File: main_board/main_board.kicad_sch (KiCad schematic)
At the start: 68 parts, among them J1 3.5mm Jack, J18 Conn_01x15_Female, J19 Conn_01x15_Female, J2 3.5mm Jack, J3 3.5mm Jack, J4 3.5mm Jack, J5 Display Header, J6 EU Power, J7 Expansion Header, SW1 Push Button, SW10 Push Button, SW11 Push Button, SW12 Push Button, SW13 Push Button, SW14 Push Button, SW15 Push Button, SW16 Push Button, SW17 Push Button, SW2 Push Button, SW3 Push Button, SW4 Push Button, SW5 Adj, SW6 Push Button, SW7 Push Button, SW8 Push Button, SW9 Push Button, U14 MCP23008-xSO, U3 CD4013BPWR, U4 CD4013BPWR

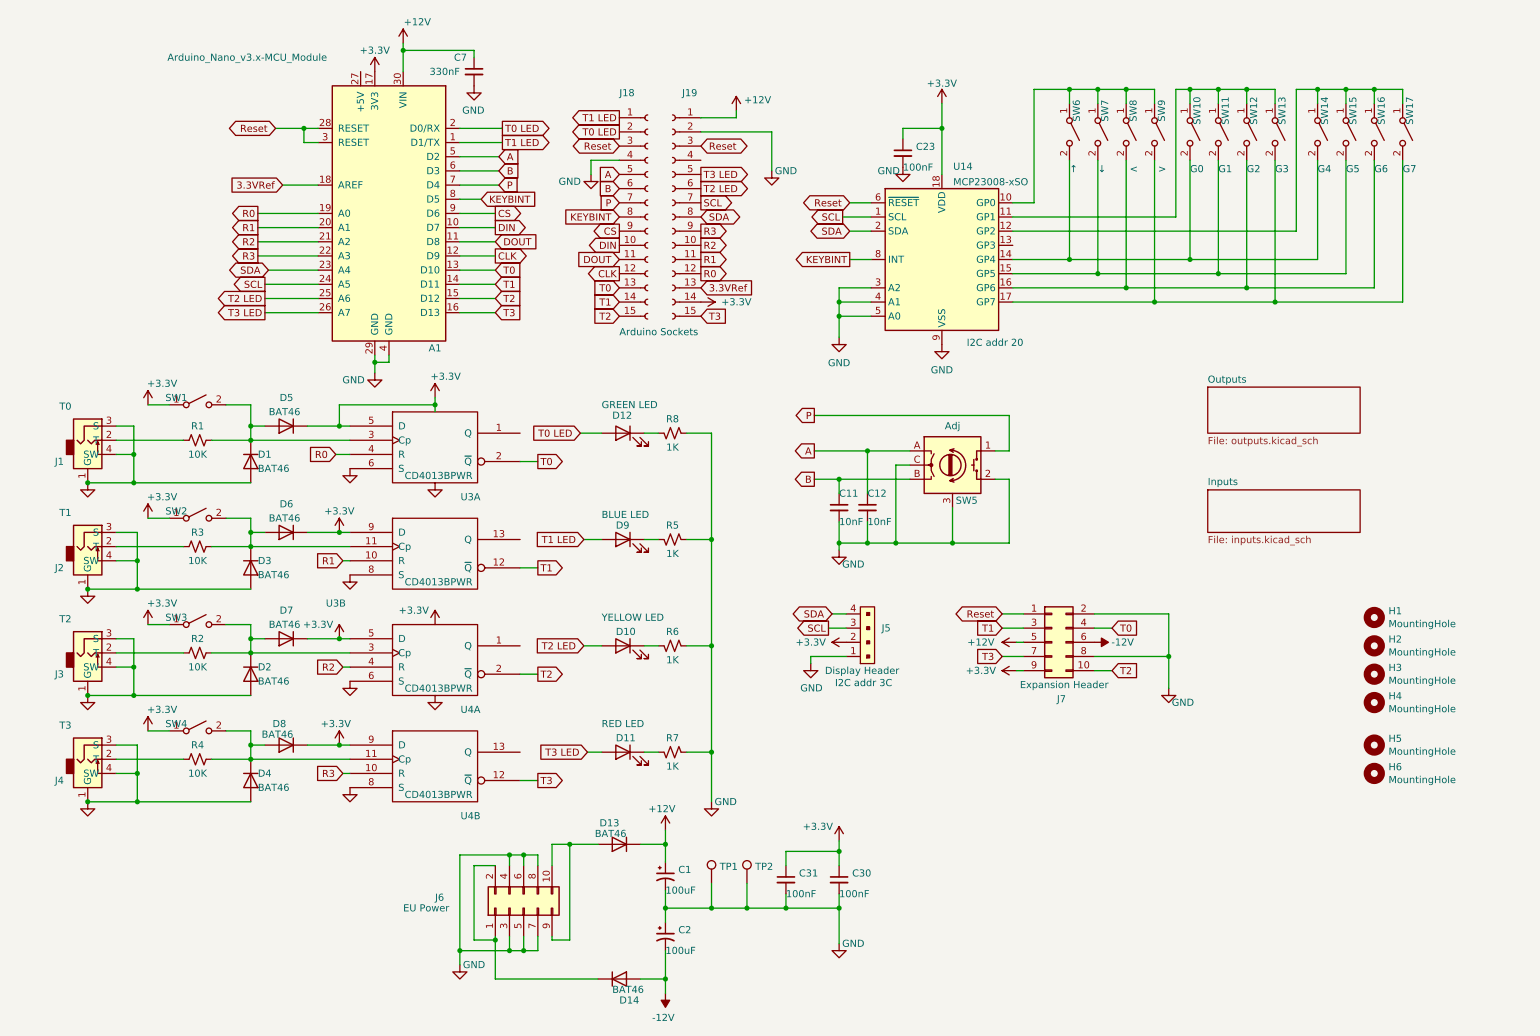
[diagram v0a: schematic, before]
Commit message: Ver 2.0 of board.
Also major advances in code.
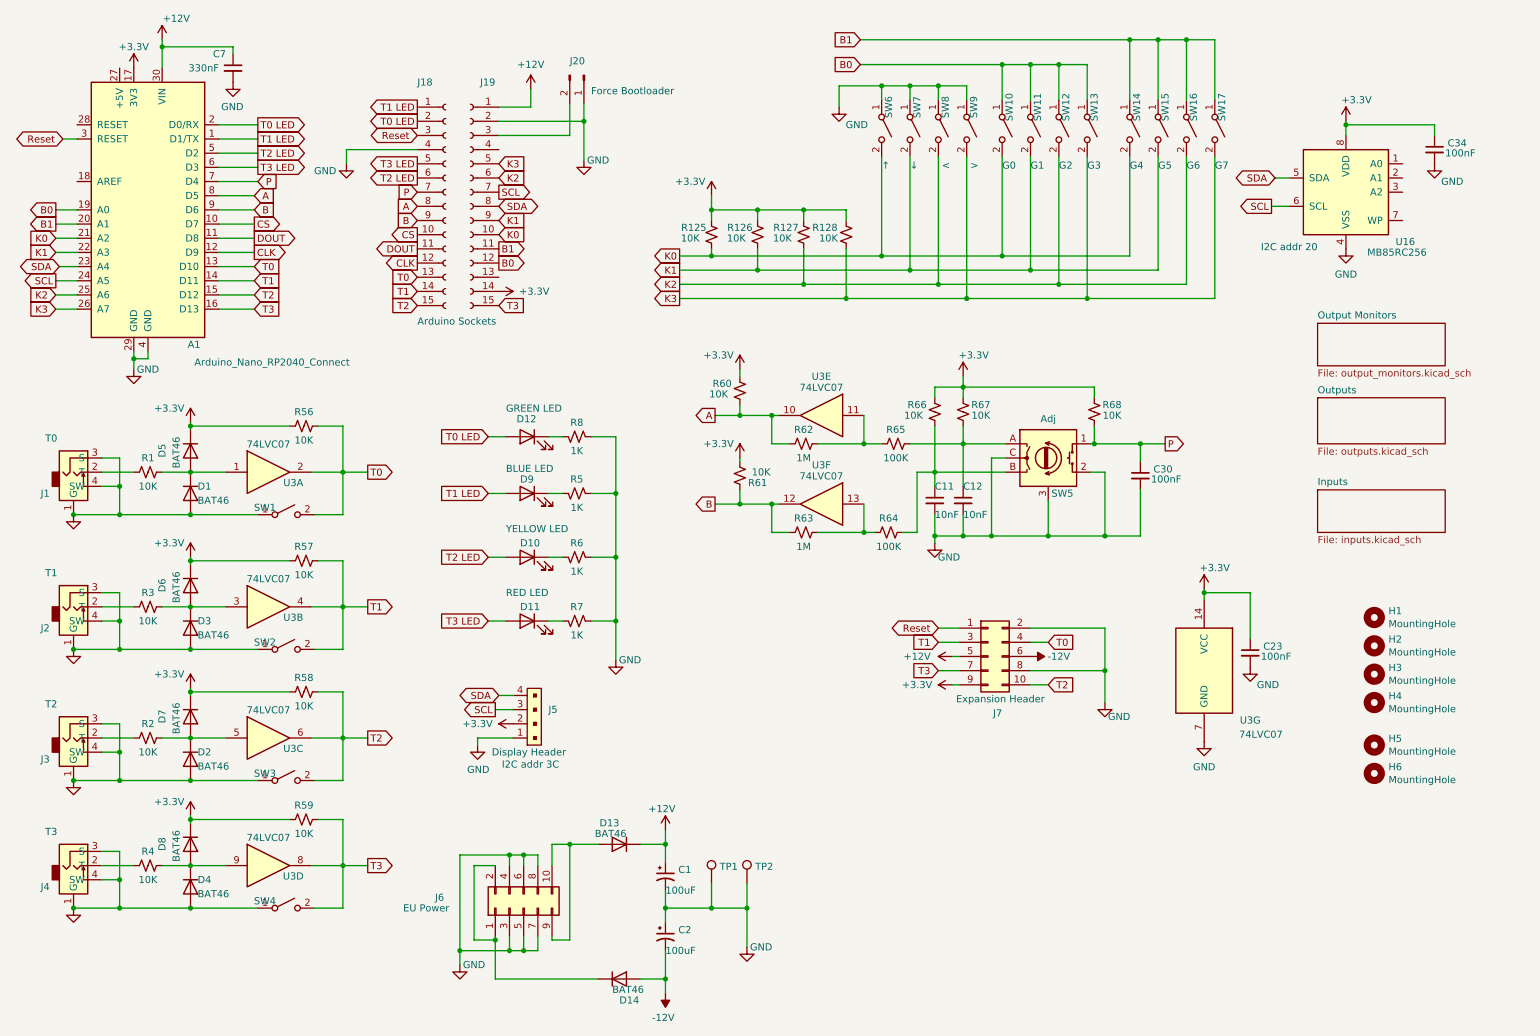
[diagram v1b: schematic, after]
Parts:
- removed C31: 100nF, Capacitor_SMD:C_0805_2012Metric_Pad1.18x1.45mm_HandSolder, symbol Device:C_Small
- removed U14: MCP23008-xSO, Package_SO:SOIC-18W_7.5x11.6mm_P1.27mm, symbol Interface_Expansion:MCP23008-xSO
- removed U3, U4: CD4013BPWR, Package_SO:TSSOP-14_4.4x5mm_P0.65mm, symbol 4xxx_IEEE:4013
- added C34: 100nF, Capacitor_SMD:C_0805_2012Metric_Pad1.18x1.45mm_HandSolder, symbol Device:C_Small
- added J20: Conn_01x02_Male, Connector_PinHeader_2.54mm:PinHeader_1x02_P2.54mm_Vertical, symbol Connector:Conn_01x02_Male
- added R125, R126, R127, R128, R56, R57, R58, R59, R60, R61, R66, R67, R68: 10K, Resistor_SMD:R_0805_2012Metric_Pad1.20x1.40mm_HandSolder, symbol Device:R_Small_US
- added R62, R63: 1M, Resistor_SMD:R_0805_2012Metric_Pad1.20x1.40mm_HandSolder, symbol Device:R_Small_US
- added R64, R65: 100K, Resistor_SMD:R_0805_2012Metric_Pad1.20x1.40mm_HandSolder, symbol Device:R_Small_US
- added U16: MB85RC256, Package_SO:SOIC-8_3.9x4.9mm_P1.27mm, symbol Memory_NVRAM:FM24C64B
- added U3: 74LVC07, Package_SO:TSSOP-14_4.4x5mm_P0.65mm, symbol 74xx:74LCX07
- A1: value Arduino_Nano_v3.x-MCU_Module -> Arduino_Nano_RP2040_Connect
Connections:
- net DIN is gone; now on net CS: A1.10 (D7), J18.10 (Pin_10)
- net KEYBINT is gone; now on net A: A1.8 (D5), J18.8 (Pin_8)
- net R0 is gone; now on net B0: A1.19 (A0), J19.12 (Pin_12)
- net R1 is gone; now on net B1: A1.20 (A1), J19.11 (Pin_11)
- net R2 is gone; now on net K0: A1.21 (A2), J19.10 (Pin_10)
- net R3 is gone; now on net K1: A1.22 (A3), J19.9 (Pin_9)
- net +3V3: now also C34.1, R125.1, R126.1, R127.1, R128.1, R56.2, R57.2, R58.2, R59.2, R60.1, R61.2, R66.1, R67.1, R68.1, U16.8 (VDD), U3.14 (VCC); no longer C30.1, SW1.1 (A), SW2.1 (A), SW3.1 (A), SW4.1 (A)
- net A: now also R60.2, R62.2, U3.10; no longer A1.5 (D2), C12.1, J18.5 (Pin_5), SW5.A
- net B: now also A1.9 (D6), J18.9 (Pin_9), R61.1, R63.2, U3.12; no longer A1.6 (D3), C11.1, J18.6 (Pin_6), SW5.B
- net CS: no longer A1.9 (D6), J18.9 (Pin_9)
- net GND: now also SW1.1 (A), SW2.1 (A), SW3.1 (A), SW4.1 (A), SW6.1 (A), SW7.1 (A), SW8.1 (A), SW9.1 (A), C34.2, J20.1 (Pin_1), U16.4 (VSS), U3.7 (GND)
- net P: now also C30.1, R68.2
- net Reset: no longer A1.28 (RESET), J19.3 (Pin_3)
- net SCL: now also U16.6 (SCL)
- net SDA: now also U16.5 (SDA)
- net T0: now also SW1.2 (B), R56.1, U3.2
- net T1: now also SW2.2 (B), R57.1, U3.4
- net T2: now also SW3.2 (B), R58.1, U3.6
- net T2 LED: now also A1.5 (D2), J18.6 (Pin_6); no longer A1.25 (A6), J19.6 (Pin_6)
- net T3: now also SW4.2 (B), R59.1, U3.8
- net T3 LED: now also A1.6 (D3), J18.5 (Pin_5); no longer A1.26 (A7), J19.5 (Pin_5)
- net at D4.1 (K), D8.2 (A), R4.1: now also U3.9; no longer SW4.2 (B)
- net B0: now reaches SW10.1 (A), SW11.1 (A), SW12.1 (A), SW13.1 (A)
- net B1: now reaches SW14.1 (A), SW15.1 (A), SW16.1 (A), SW17.1 (A)
- net K0: now reaches SW10.2 (B), SW14.2 (B), SW6.2 (B)
- net K0: now also R125.2
- net K1: now reaches SW11.2 (B), SW15.2 (B), SW7.2 (B)
- net K1: now also R126.2
- net K2: now reaches SW12.2 (B), SW16.2 (B), SW8.2 (B)
- net K2: now also A1.25 (A6), J19.6 (Pin_6), R127.2
- net K3: now reaches SW13.2 (B), SW17.2 (B), SW9.2 (B)
- net K3: now also A1.26 (A7), J19.5 (Pin_5), R128.2
- net at D2.1 (K), D7.2 (A), R2.1: now also U3.5; no longer SW3.2 (B)
- net at D3.1 (K), D6.2 (A), R3.1: now also U3.3; no longer SW2.2 (B)
- net at D1.1 (K), D5.2 (A), R1.1: now also U3.1; no longer SW1.2 (B)
- net 3.3VRef: no longer names the net of A1.18 (AREF)
- net 3.3VRef: no longer J19.13 (Pin_13)
- new net: C12.1, R65.1, R67.2, SW5.A
- new net: R63.1, R64.2, U3.13
- new net: R62.1, R65.2, U3.11
- new net: J19.3 (Pin_3), J20.2 (Pin_2)
- new net: C11.1, R64.1, R66.2, SW5.B
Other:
- added sheet Output Monitors (output_monitors.kicad_sch)
- note added: "Force Bootloader"
- moved on the sheet: A1, C11, C12, C7, D1, D10, D11, D12, D5, D9, J1, J18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
